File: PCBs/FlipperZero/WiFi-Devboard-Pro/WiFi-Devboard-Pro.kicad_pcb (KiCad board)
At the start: 2 copper layers, 78.5 x 20.1 mm, 46 parts, among them IC1 ESP32-WROOM-32E-N4, IC2 DMP1045U-7, IC3 AZ1117H-3.3TRE1, IC4 DMP1045U-7, IC5 DMP1045U-7, J1 3220-10-0300-00, J2 X6511WVS-08H-C60D48R2, J3 DZ254S-11-10-48, J4 Conn_01x11, J5 Conn_01x11, J6 503398-1892, U1 MMDT2907A-7-F, U2 MMDT2907A-7-F, U3 MMDT2907A-7-F

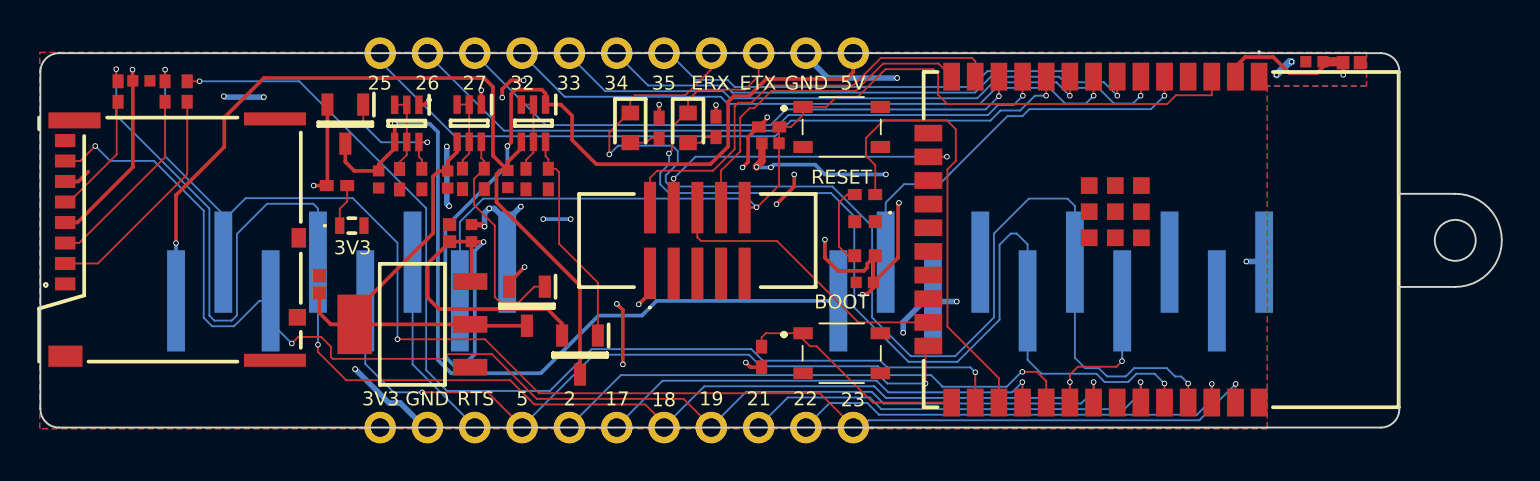
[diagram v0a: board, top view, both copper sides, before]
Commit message: started review
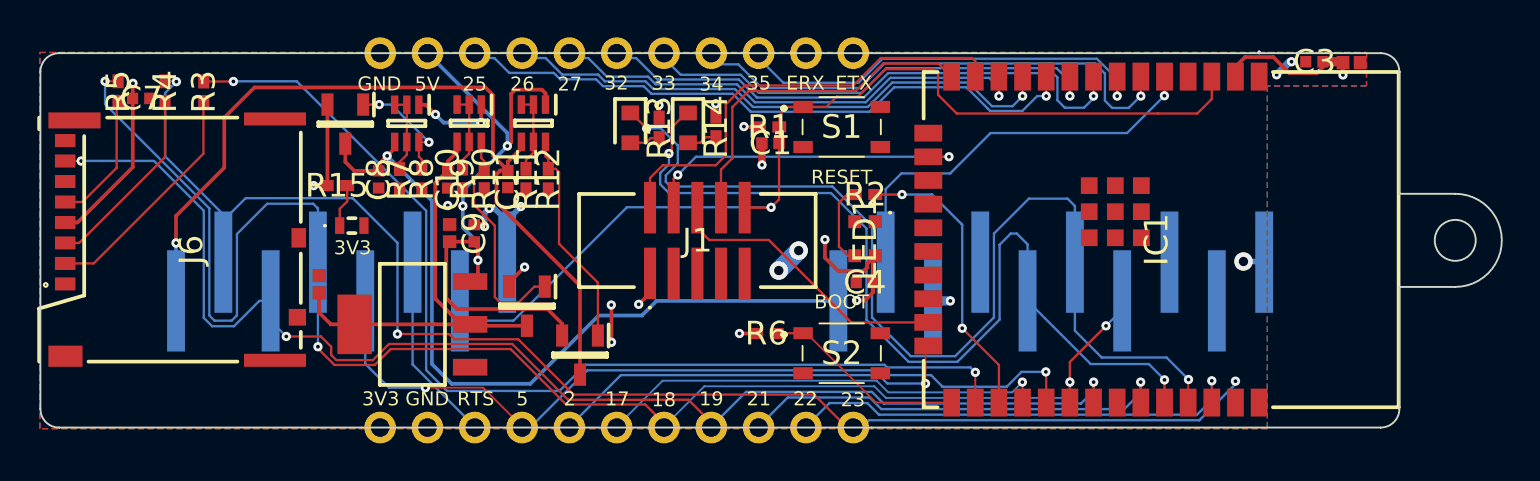
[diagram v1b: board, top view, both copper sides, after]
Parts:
- moved R6 1.29 mm to (150.1, 104.9), turned to 180 degrees
- moved C7 0.95 mm to (116.5, 92.3)
- moved R3 0.89 mm to (119.9, 91.9)
- moved C9 0.15 mm to (134.4, 99.5)
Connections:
- J4 pad 1: +3V3 -> GND
- J4 pad 2: GND -> +3V3
- J5 pad 1: GPIO25 -> GND
- J5 pad 10: GND -> RX
- J5 pad 11: +5V -> TX
- J5 pad 2: GPIO26 -> +5V
- J5 pad 3: GPIO27 -> GPIO25
- J5 pad 4: GPIO32 -> GPIO26
- J5 pad 5: GPIO33 -> GPIO27
- J5 pad 6: GPIO34 -> GPIO32
- J5 pad 7: GPIO35 -> GPIO33
- J5 pad 8: RX -> GPIO34
- J5 pad 9: TX -> GPIO35
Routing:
- net +5V: track 65.4 -> 33.9 mm, vias 2 -> 3
- net GND: track 42.1 -> 14.5 mm, vias 19 -> 11
- net RX: track 66.4 -> 55.6 mm
- net +3V3: track 53.0 -> 43.9 mm, vias 21 -> 15
- net GPIO16: track 24.7 -> 15.7 mm, vias 0 -> 2
- net TX: track 58.2 -> 49.9 mm
- net GPIO25: track 39.7 -> 34.3 mm
- net GPIO26: track 35.5 -> 30.3 mm
- net GPIO27: track 31.4 -> 26.3 mm
- net GPIO33: track 29.6 -> 25.2 mm
- net GPIO35: track 27.0 -> 22.7 mm
- net GPIO32: track 33.7 -> 29.9 mm
- net GPIO34: track 31.1 -> 27.4 mm
- net +ext_3V3: track 44.0 -> 41.1 mm
- net GPIO04: track 57.4 -> 55.7 mm
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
